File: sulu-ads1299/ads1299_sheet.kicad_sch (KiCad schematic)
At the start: 15 parts, among them U4 ADS1299_TQFP-64

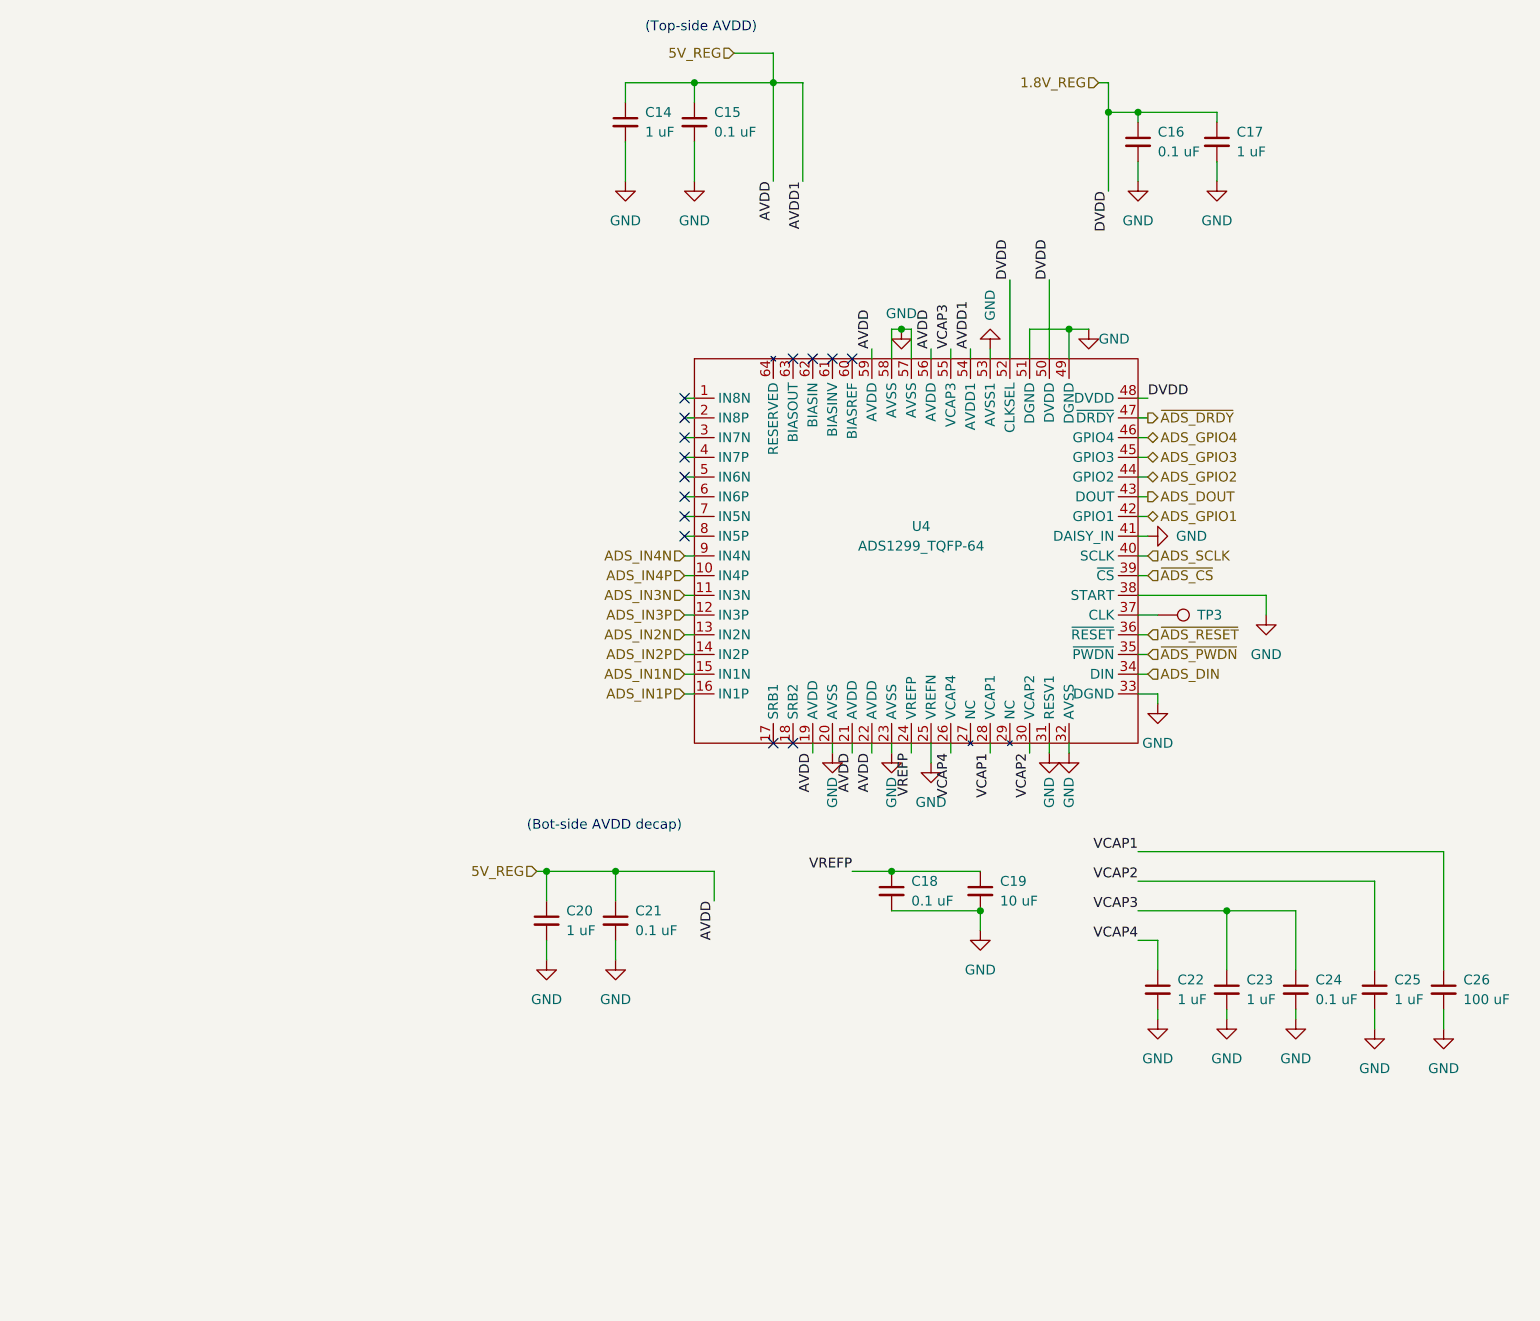
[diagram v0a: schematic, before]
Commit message: DRC clean layout of Rev. 3
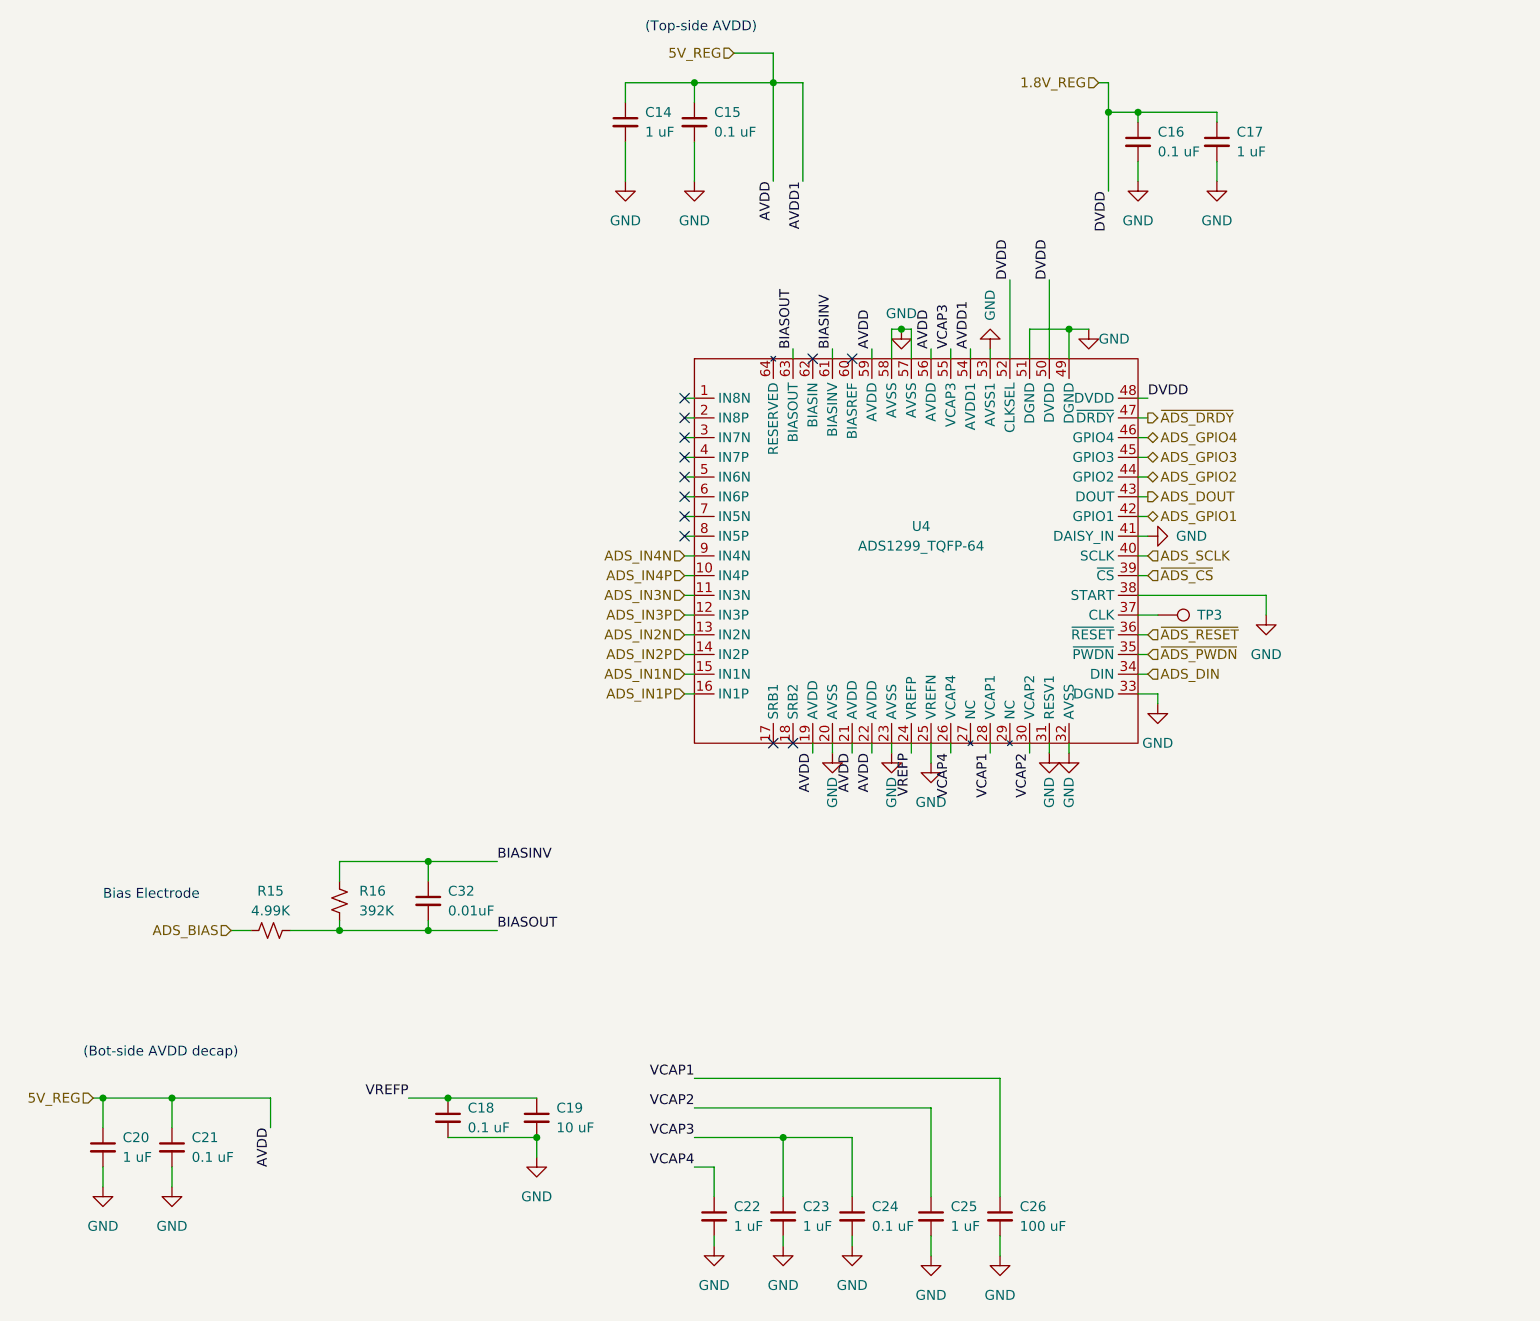
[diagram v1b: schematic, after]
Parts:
- added C32: 0.01uF, Capacitor_SMD:C_0603_1608Metric, symbol Device:C_Small
- added R15: 4.99K, Resistor_SMD:R_0603_1608Metric, symbol Device:R_Small_US
- added R16: 392K, Resistor_SMD:R_0603_1608Metric, symbol Device:R_Small_US
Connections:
- net BIASINV: now reaches U4.61 (BIASINV)
- net BIASINV: now also C32.1, R16.1
- net BIASOUT: now reaches U4.63 (BIASOUT)
- net BIASOUT: now also C32.2, R15.2, R16.2
- new net ADS_BIAS: R15.1
- no-connect marks 14 -> 12
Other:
- note added: "Bias Electrode"
- moved on the sheet: C18, C19, C20, C21, C22, C23, C24, C25, C26
